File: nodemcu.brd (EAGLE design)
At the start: 47.9 x 48.2 mm, 8 parts

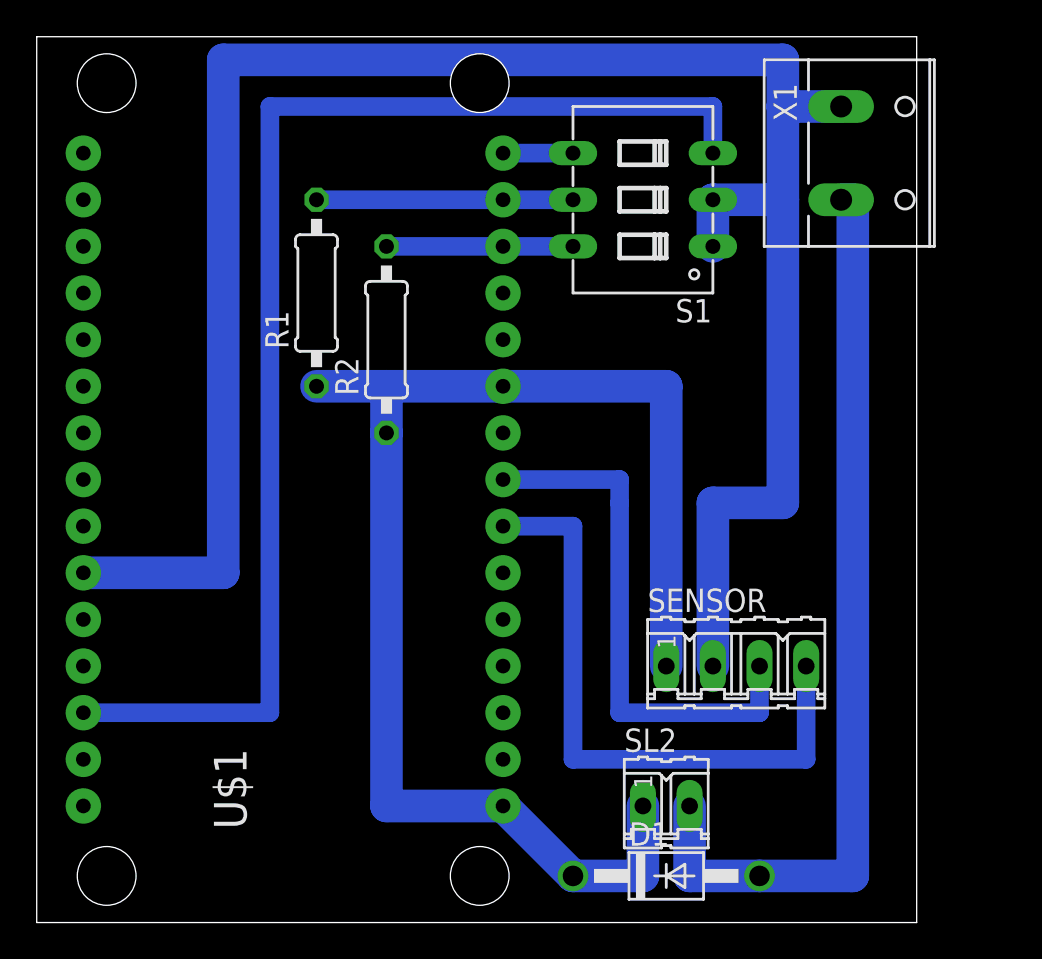
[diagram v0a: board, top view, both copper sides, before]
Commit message: uprava desky
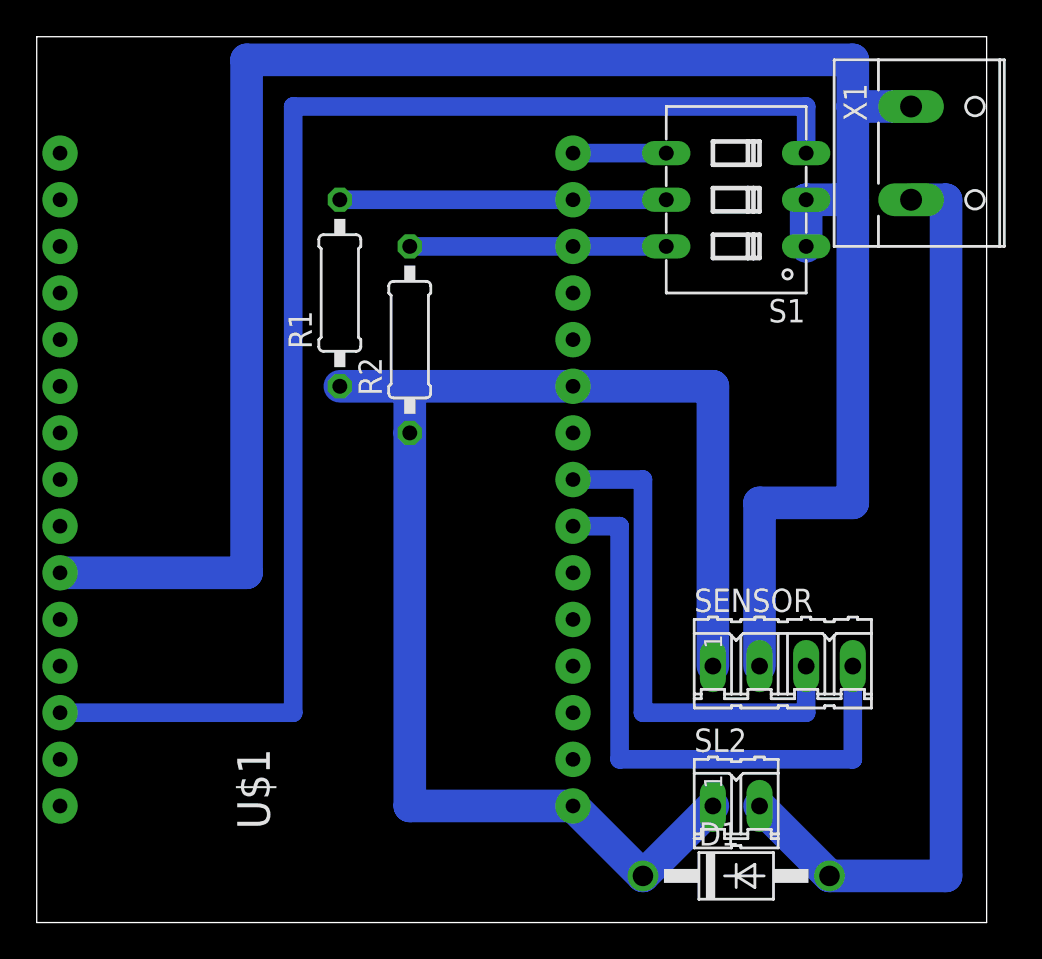
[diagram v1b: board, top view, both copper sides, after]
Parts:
- moved S1 5.08 mm to (38.1, 39.4)
- moved D1 3.81 mm to (38.1, 2.54)
- moved SL2 3.81 mm to (38.1, 6.35)
- moved U$1 3.81 mm to (17.8, 24.1)
- moved X1 3.81 mm to (48.3, 41.9)
- moved SENSOR 2.54 mm to (40.6, 14.0)
- moved R1 1.27 mm to (16.5, 34.3)
- moved R2 1.27 mm to (20.3, 31.8)
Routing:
- net N$4: track 69.9 -> 76.2 mm
- net GND: track 112.4 -> 117.5 mm
- net N$9: track 10.2 -> 14.0 mm
- net N$8: track 14.0 -> 17.8 mm
- net +3V3: track 76.5 -> 78.1 mm
- net N$3: track 29.2 -> 27.9 mm
- net N$2: track 34.3 -> 33.0 mm
- net N$1: track 3.81 -> 5.08 mm
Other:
- board size 47.9 x 48.2 mm -> 51.7 x 48.2 mm
